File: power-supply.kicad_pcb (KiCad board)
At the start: 2 copper layers, 100 x 100 mm, 89 parts, among them J1 KRE, J10 KRE, J11 Fan, J14 I2C, J2 Conn_01x05, J5 Conn_01x20, J7 Conn_01x20, K1 Rele 5V, K2 Rele 5V, Q3 IRF740, Q4 MMBT3904, Q5 MMBT3904, Q6 MMBT3904, U1 LM324, U2 LMV7219M5, U3 TC4427, U4 AMS1117-5.0, U5 74HC00, U6 74LVC1G08, U7 AMS1117-3.3

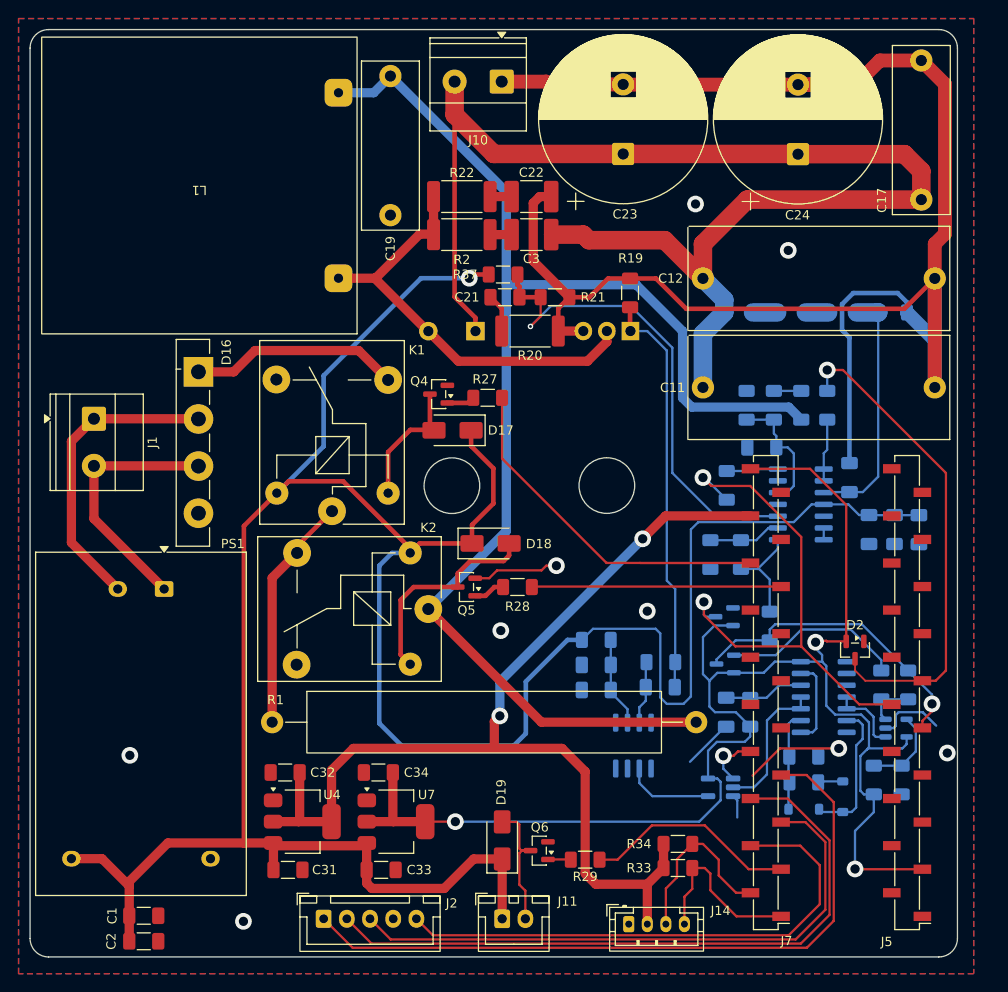
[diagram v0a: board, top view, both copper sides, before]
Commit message: pcb: atualizar layout 2D da placa e esquematicos
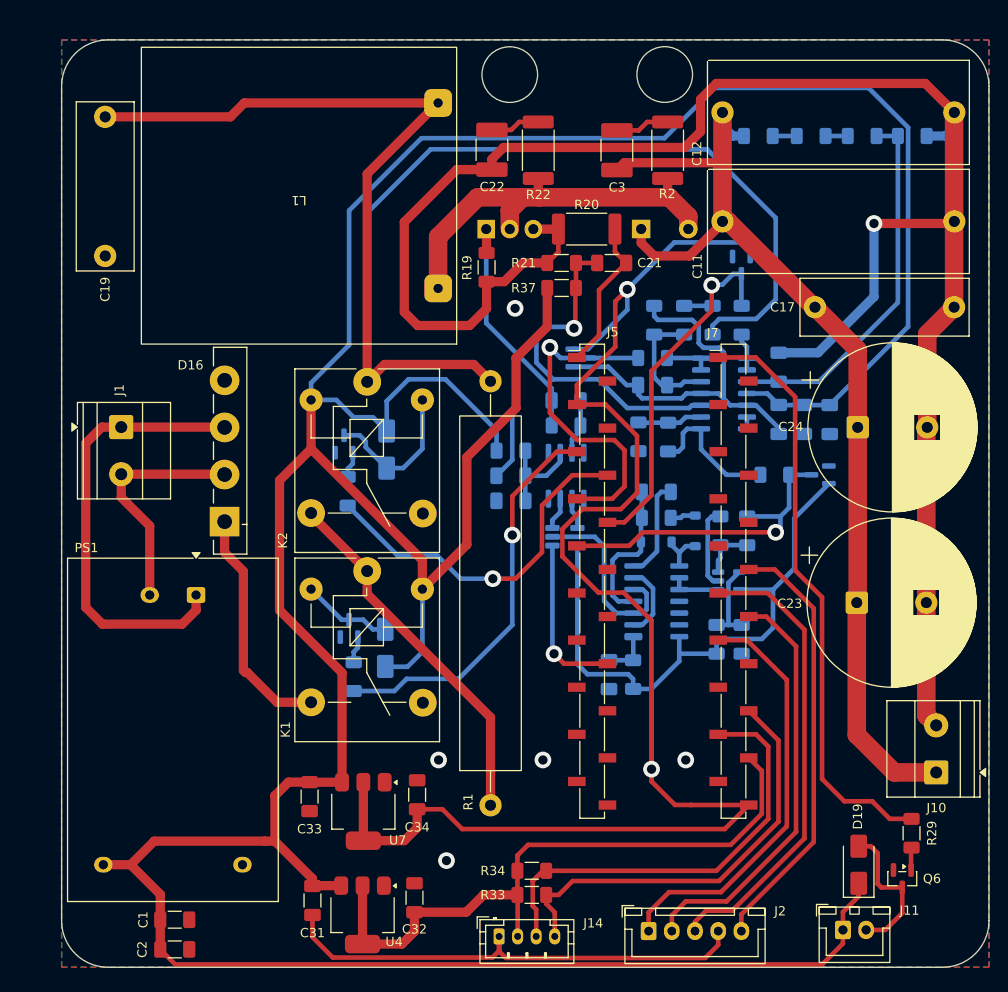
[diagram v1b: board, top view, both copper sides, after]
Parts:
- D17, D18, D2, Q4, Q5, R27, R28: moved to B.Cu
- moved J10 88.0 mm to (199.3, 124.0), turned to 90 degrees
- moved C23 54.5 mm to (190.7, 105.7), turned to 0 degrees
- moved D2 43.3 mm to (178.3, 69.3)
- moved Q6 39.3 mm to (195.7, 135.4), turned to -90 degrees
- moved D19 38.5 mm to (190.9, 133.9)
- moved J11 36.8 mm to (189.2, 141.0)
- moved J5 36.0 mm to (162.2, 103.4), turned to 0 degrees
- moved R29 35.3 mm to (196.7, 130.6), turned to -90 degrees
- moved J2 35.1 mm to (168.3, 141.1)
- moved R27 33.4 mm to (136.5, 113.7), turned to -90 degrees
- moved D6 32.9 mm to (169.1, 99.1)
- moved D5 32.8 mm to (173.3, 97.9)
- moved C4 32.7 mm to (169.1, 93.7)
- moved R6 32.7 mm to (169.1, 96.5)
- moved C28 32.5 mm to (159.4, 83.9), turned to 180 degrees
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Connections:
- D2 pad 3: /MCU/PA5 -> /MCU/PB0
- D3 pad 3: /MCU/PA6 -> /MCU/PB1
- J1 pad 1: /N -> /L
- J1 pad 2: /L -> /N
- J10 pad 1: /PFC/GND_380V -> /PFC/DC_380V
- J10 pad 2: /PFC/DC_380V -> /PFC/GND_380V
- J14 pad 3: /MCU/PB13 -> /MCU/PB9
- J14 pad 4: /MCU/PB12 -> /MCU/PB8
- J2 pad 1: /MCU/PA10 -> /MCU/PB5
- J2 pad 2: /MCU/PA9 -> /MCU/PB4
- J2 pad 3: /MCU/PA8 -> /MCU/PB3
- J2 pad 5: /MCU/PB15 -> /MCU/PA15
- R27 pad 2: /MCU/PB8 -> /MCU/PB11
- R28 pad 2: /MCU/PB7 -> /MCU/PB10
- R29 pad 1: /MCU/PB14 -> /MCU/PB12
- R33 pad 2: /MCU/PB12 -> /MCU/PB8
- R34 pad 2: /MCU/PB13 -> /MCU/PB9
- R39 pad 2: /MCU/PA5 -> /MCU/PB0
- R40 pad 2: /MCU/PA6 -> /MCU/PB1
- U5 pad 1: unconnected-(U5-Pad1) -> /PFC/RESET_OC
- U5 pad 10: /PFC/ENABLE -> Net-(U2-Pad1)
- U5 pad 11: /PFC/ENABLE -> unconnected-(U5-Pad11)
- U5 pad 12: /PFC/RESET_OC -> unconnected-(U5-Pad12)
- U5 pad 13: Net-(U5-Pad13) -> unconnected-(U5-Pad13)
- U5 pad 2: unconnected-(U5-Pad2) -> Net-(U5-Pad2)
- U5 pad 3: unconnected-(U5-Pad3) -> /PFC/ENABLE
- U5 pad 4: Net-(U2-Pad1) -> Net-(D6-A)
- U5 pad 5: Net-(U2-Pad1) -> /PFC/ENABLE
- U5 pad 6: Net-(D5-A) -> Net-(U5-Pad2)
- U5 pad 8: Net-(U5-Pad13) -> Net-(D5-A)
- U5 pad 9: Net-(D6-A) -> Net-(U2-Pad1)
- U6 pad 1: /MCU/PA11 -> /MCU/PA2
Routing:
- net +12V: track 303.7 -> 412.4 mm, vias 1 -> 0
- net GND_311V: track 58.9 -> 143.5 mm, vias 9 -> 5
- net /MCU/PA10: track 77.2 -> 0.00 mm
- net /MCU/PA9: track 72.9 -> 0.00 mm
- net +3V3: track 160.5 -> 233.1 mm, vias 3 -> 2
- net /MCU/PA8: track 64.3 -> 0.00 mm
- net /MCU/PB15: track 58.2 -> 0.00 mm
- net /MCU/PA6: track 57.0 -> 0.00 mm, vias 2 -> 0
- net /MCU/PA5: track 52.9 -> 0.00 mm, vias 1 -> 0
- net /MCU/PB3: track 0.00 -> 50.4 mm
- net /MCU/PB9: track 0.00 -> 48.1 mm
- net /MCU/PA15: track 0.00 -> 46.8 mm
- net +5V: track 116.0 -> 70.0 mm, vias 2 -> 0
- net /MCU/PB5: track 0.00 -> 45.7 mm
- net /MCU/PB4: track 0.00 -> 45.3 mm
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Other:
- outline, holes or cut-outs redrawn
